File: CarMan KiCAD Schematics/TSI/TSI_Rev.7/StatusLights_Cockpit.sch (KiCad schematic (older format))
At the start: 17 parts, among them SW4 RTDS Test, U1 RDE03110S12, U11 TLP293, U13 TLP293, U43 NCD9830DBR2G

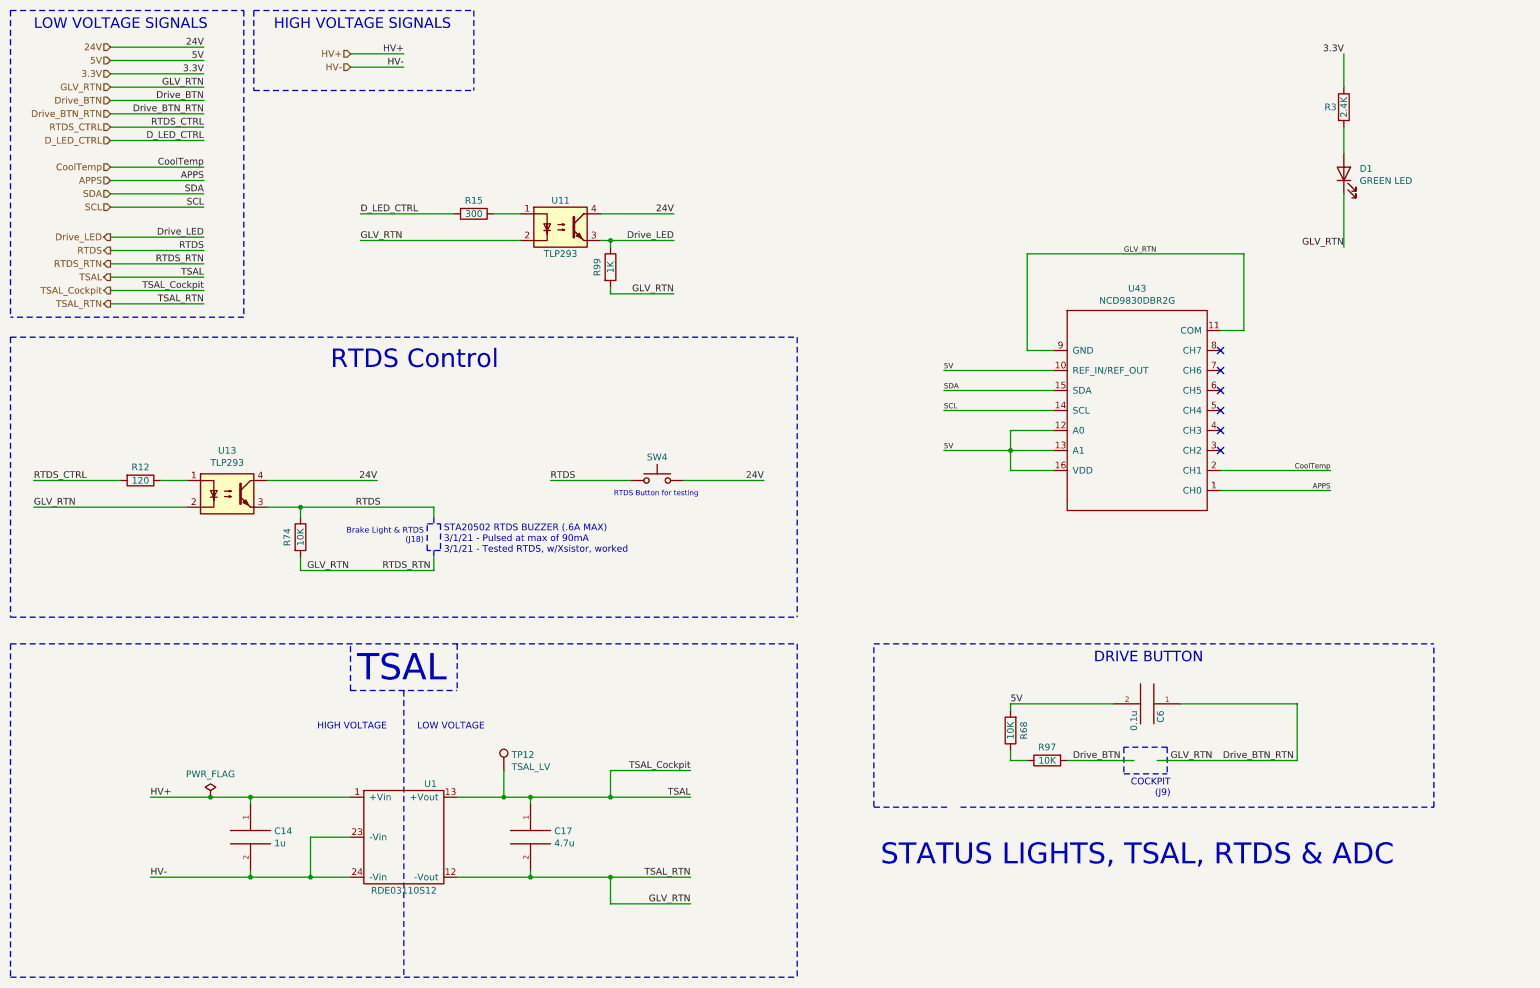
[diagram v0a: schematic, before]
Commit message: TSI Should be final schematic
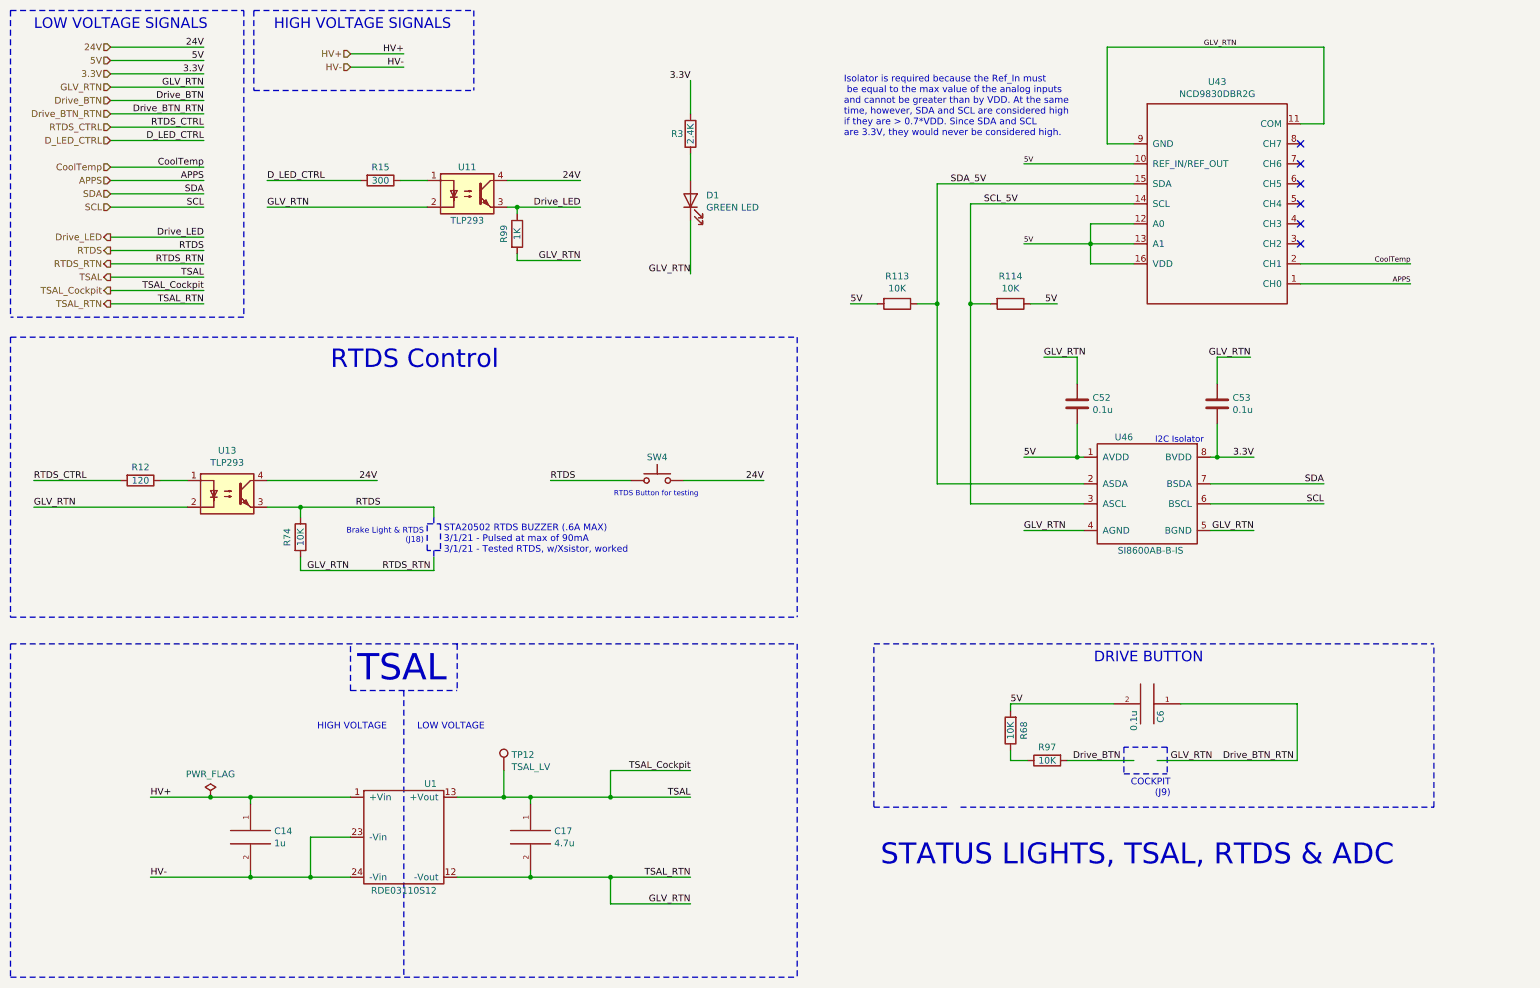
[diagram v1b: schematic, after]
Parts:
- added C52, C53: 0.1u, Capacitor_SMD:C_0805_2012Metric_Pad1.18x1.45mm_HandSolder, symbol Device:C
- added R113, R114: 10K, Resistor_SMD:R_0805_2012Metric_Pad1.20x1.40mm_HandSolder, symbol Device:R
- added U46: SI8600AB-B-IS, TSI_Rev_2021_Footprint_Lib:SOIC127P600X175-8N, symbol CarMan_KiCAD_Library:SI8600AB-B-IS
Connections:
- net labels added: SCL_5V, SDA_5V
- wire segments 93 -> 117
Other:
- note added: "I2C Isolator\n"
- note added: "Isolator is required because the Ref_In must\n be equal to the max value of the analog inputs \nand cannot be greater than by VDD. At the same\ntime, however, SDA and SCL are considered high \nif they are > 0.7*VDD. Since SDA and SCL \nare 3.3V, they would never be considered high."
- moved on the sheet: D1, R15, R3, R99, U11, U43

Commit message: Pre-review_schematic
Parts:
- C17, C6: footprint Capacitor_SMD:C_0805_2012Metric_Pad1.15x1.40mm_HandSolder -> Capacitor_SMD:C_0805_2012Metric_Pad1.18x1.45mm_HandSolder
- R12, R15, R3, R68, R74, R97, R99: footprint Resistor_SMD:R_0805_2012Metric_Pad1.15x1.40mm_HandSolder -> Resistor_SMD:R_0805_2012Metric_Pad1.20x1.40mm_HandSolder
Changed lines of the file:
@@
 F 0 "R3" H 5500 1425 50  0000 C CNN
 F 1 "2.4K" V 5600 1425 50  0000 C CNN
-F 2 "Resistor_SMD:R_0805_2012Metric_Pad1.15x1.40mm_HandSolder" V 5530 1425 50  0001 C CNN
+F 2 "Resistor_SMD:R_0805_2012Metric_Pad1.20x1.40mm_HandSolder" V 5530 1425 50  0001 C CNN
 F 3 "~" H 5600 1425 50  0001 C CNN
 	1    5600 1425
@@
 F 0 "R15" V 3175 1775 50  0000 C CNN
 F 1 "300" V 3275 1775 50  0000 C CNN
-F 2 "Resistor_SMD:R_0805_2012Metric_Pad1.15x1.40mm_HandSolder" V 3205 1775 50  0001 C CNN
+F 2 "Resistor_SMD:R_0805_2012Metric_Pad1.20x1.40mm_HandSolder" V 3205 1775 50  0001 C CNN
 F 3 "~" H 3275 1775 50  0001 C CNN
 	1    3275 1775
@@
 F 0 "C17" H 4578 6746 50  0000 L CNN
 F 1 "4.7u" H 4578 6655 50  0000 L CNN
-F 2 "Capacitor_SMD:C_0805_2012Metric_Pad1.15x1.40mm_HandSolder" H 4400 6700 50  0001 C CNN
+F 2 "Capacitor_SMD:C_0805_2012Metric_Pad1.18x1.45mm_HandSolder" H 4400 6700 50  0001 C CNN
 F 3 "~" H 4400 6700 50  0001 C CNN
 	1    4400 6700
@@
 F 0 "C6" H 9075 5800 50  0000 L CNN
 F 1 "0.1u" H 9075 5600 50  0000 L CNN
-F 2 "Capacitor_SMD:C_0805_2012Metric_Pad1.15x1.40mm_HandSolder" H 9025 5700 50  0001 C CNN
+F 2 "Capacitor_SMD:C_0805_2012Metric_Pad1.18x1.45mm_HandSolder" H 9025 5700 50  0001 C CNN
 F 3 "~" H 9025 5700 50  0001 C CNN
 	1    9025 5700
@@
 F 0 "R97" V 8175 6125 50  0000 C CNN
 F 1 "10K" V 8275 6125 50  0000 C CNN
-F 2 "Resistor_SMD:R_0805_2012Metric_Pad1.15x1.40mm_HandSolder" V 8205 6125 50  0001 C CNN
+F 2 "Resistor_SMD:R_0805_2012Metric_Pad1.20x1.40mm_HandSolder" V 8205 6125 50  0001 C CNN
 F 3 "~" H 8275 6125 50  0001 C CNN
 	1    8275 6125
@@
 F 0 "R74" V 2575 4450 50  0000 C CNN
 F 1 "10K" V 2675 4450 50  0000 C CNN
-F 2 "Resistor_SMD:R_0805_2012Metric_Pad1.15x1.40mm_HandSolder" V 2605 4450 50  0001 C CNN
+F 2 "Resistor_SMD:R_0805_2012Metric_Pad1.20x1.40mm_HandSolder" V 2605 4450 50  0001 C CNN
 F 3 "~" H 2675 4450 50  0001 C CNN
 	1    2675 4450
@@
 F 0 "R12" V 1375 4025 50  0000 C CNN
 F 1 "120" V 1475 4025 50  0000 C CNN
-F 2 "Resistor_SMD:R_0805_2012Metric_Pad1.15x1.40mm_HandSolder" V 1405 4025 50  0001 C CNN
+F 2 "Resistor_SMD:R_0805_2012Metric_Pad1.20x1.40mm_HandSolder" V 1405 4025 50  0001 C CNN
 F 3 "~" H 1475 4025 50  0001 C CNN
 	1    1475 4025
@@
 F 0 "R68" V 7900 5900 50  0000 C CNN
 F 1 "10K" V 8000 5900 50  0000 C CNN
-F 2 "Resistor_SMD:R_0805_2012Metric_Pad1.15x1.40mm_HandSolder" V 7930 5900 50  0001 C CNN
+F 2 "Resistor_SMD:R_0805_2012Metric_Pad1.20x1.40mm_HandSolder" V 7930 5900 50  0001 C CNN
 F 3 "~" H 8000 5900 50  0001 C CNN
 	1    8000 5900
@@
 F 0 "R99" V 4200 2175 50  0000 C CNN
 F 1 "1K" V 4300 2175 50  0000 C CNN
-F 2 "Resistor_SMD:R_0805_2012Metric_Pad1.15x1.40mm_HandSolder" V 4230 2175 50  0001 C CNN
+F 2 "Resistor_SMD:R_0805_2012Metric_Pad1.20x1.40mm_HandSolder" V 4230 2175 50  0001 C CNN
 F 3 "~" H 4300 2175 50  0001 C CNN
 	1    4300 2175
